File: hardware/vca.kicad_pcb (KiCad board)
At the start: 2 copper layers, 76.2 x 109.2 mm, 93 parts, among them P1 VCA_CMD_PWR, P10 CARD_2, P11 OUT_MAIN, P12 OUT_GND, P2 CARD_0, P3 CARD_1, P4 OUT_0, P5 OUT_1, P6 OUT_2, P7 OUT_3, P8 OUT_4, P9 OUT_5, U1 TL074, U10 TL082, U2 TL082, U3 4051, U4 SSM2164, U5 TL082, U6 TL082, U7 TL074, U8 SSM2164, U9 TL082

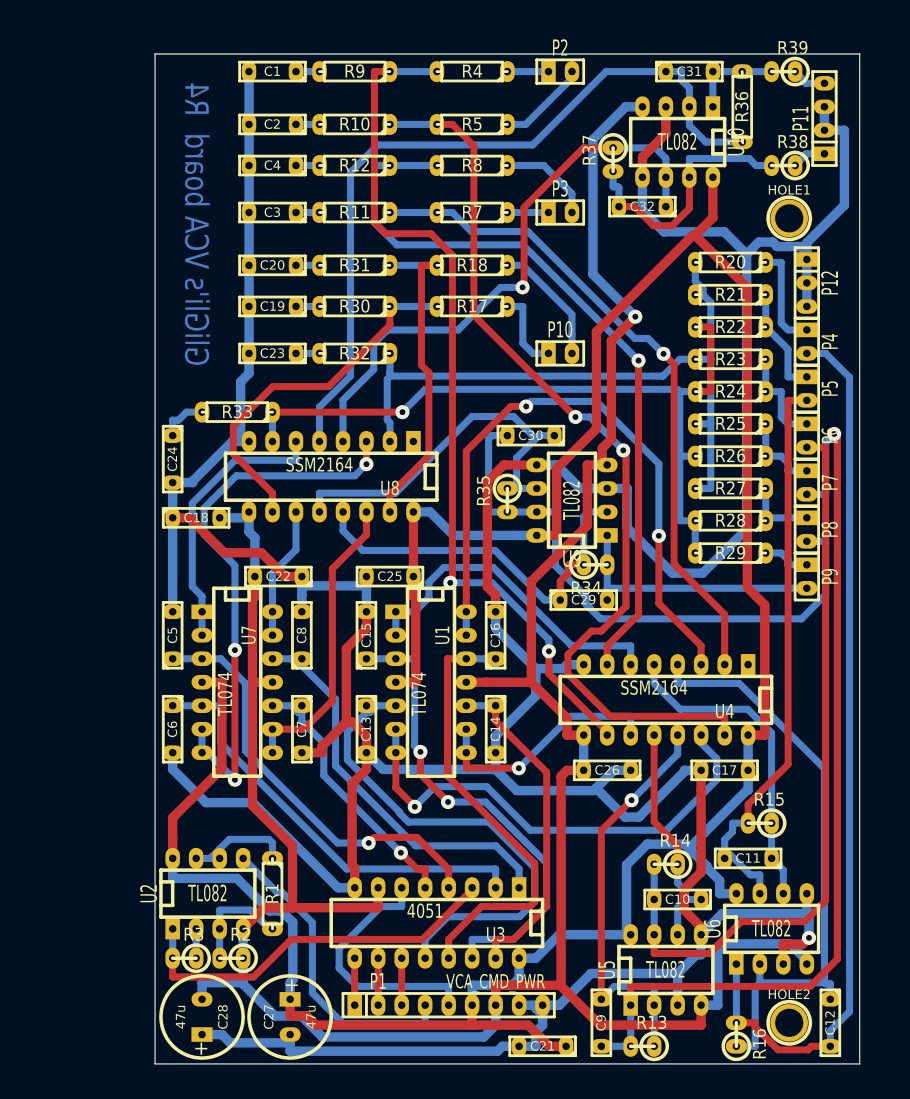
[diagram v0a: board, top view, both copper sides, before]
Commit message: hw: LM13700 vca board wip
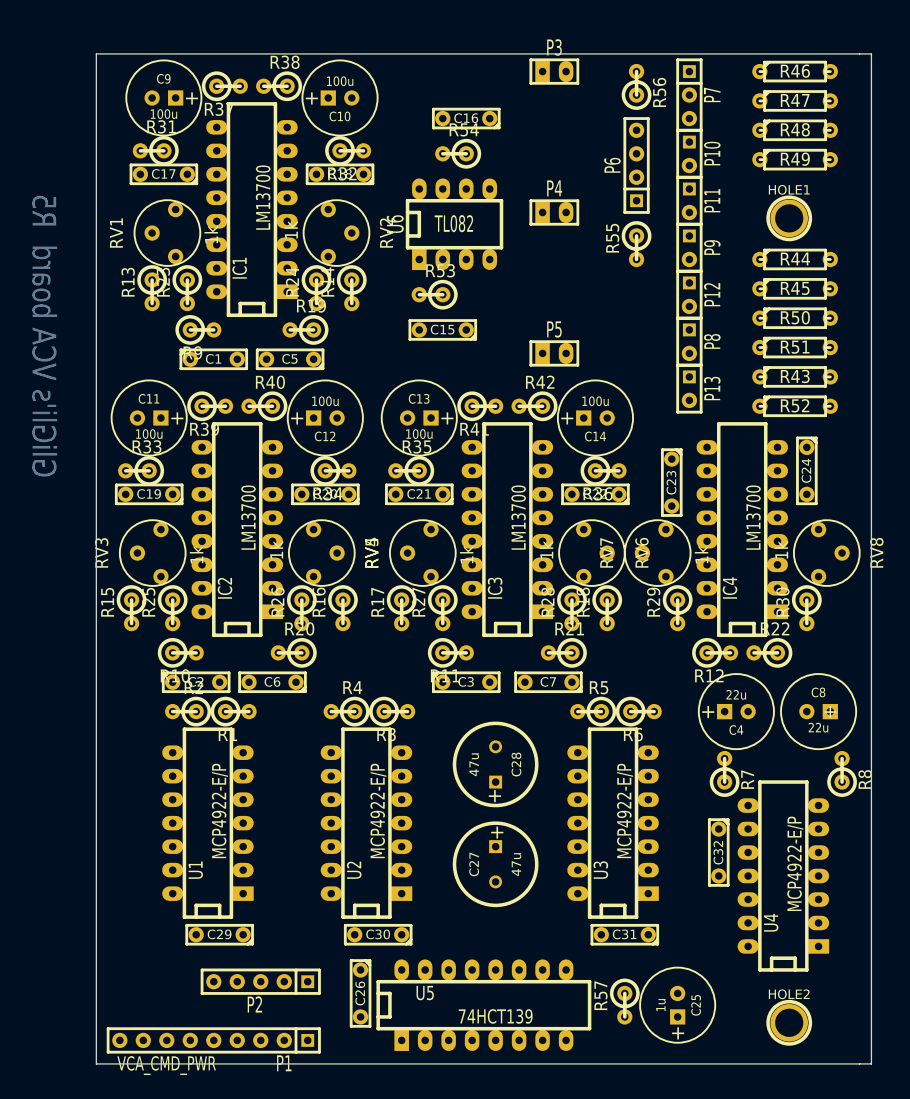
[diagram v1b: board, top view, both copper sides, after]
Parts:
- removed U10, U9: TL082, DIP-8__300_ELL
- removed U7: TL074, DIP-14__300_ELL
- removed U8: SSM2164, DIP-16__300_ELL
- added IC1: LM13700, DIP-16__300_ELL, F.Cu at (89.2, 67.6)
- added IC2: LM13700, DIP-16__300_ELL, F.Cu at (87.6, 102.2)
- added IC3: LM13700, DIP-16__300_ELL, F.Cu at (116.8, 102.2)
- added IC4: LM13700, DIP-16__300_ELL, F.Cu at (142.2, 102.2)
- added P13: OUT_5, SIL-2, F.Cu at (136.5, 87.0)
- added R19: 1k, R1, F.Cu at (94.6, 80.6)
- added R40: 4k7, R1, F.Cu at (90.2, 88.9)
- added R41: 4k7, R1, F.Cu at (114.3, 88.9)
- added R42: 4k7, R1, F.Cu at (119.4, 88.9)
- added R43: 33k, R3-LARGE_PADS, F.Cu at (148.0, 85.7)
- added R44: 47k, R3-LARGE_PADS, F.Cu at (148.0, 73.0)
- added R45: 150k, R3-LARGE_PADS, F.Cu at (148.0, 76.2)
- added R46: 56k, R3-LARGE_PADS, F.Cu at (148.0, 52.7)
- added R47: 68k, R3-LARGE_PADS, F.Cu at (148.0, 55.9)
- added R48: 68k, R3-LARGE_PADS, F.Cu at (148.0, 59.1)
- added R49: 56k, R3-LARGE_PADS, F.Cu at (148.0, 62.2)
- added R50: 150k, R3-LARGE_PADS, F.Cu at (148.0, 79.4)
- added R51: 47k, R3-LARGE_PADS, F.Cu at (148.0, 82.5)
- added R52: 33k, R3-LARGE_PADS, F.Cu at (148.0, 88.9)
- added R53: 47k, R1, F.Cu at (108.6, 76.8)
- added R54: 47k, R1, F.Cu at (111.1, 61.6)
- added R55: 1k, R1, F.Cu at (130.8, 71.8)
- added R56: 1k, R1, F.Cu at (130.8, 54.0)
- added R57: 100k, R1, F.Cu at (129.5, 153.7)
- added R6: 4k7, R1, F.Cu at (131.4, 121.9)
- added RV1: 1k, RV2, F.Cu at (79.7, 70.2)
- added RV2: 1k, RV2, F.Cu at (98.7, 70.2)
- added RV3: 1k, RV2, F.Cu at (78.1, 104.8)
- added RV4: 1k, RV2, F.Cu at (97.2, 104.8)
- added RV5: 1k, RV2, F.Cu at (107.3, 104.8)
- added RV6: 1k, RV2, F.Cu at (126.4, 104.8)
- added RV7: 1k, RV2, F.Cu at (132.7, 104.8)
- added RV8: 1k, RV2, F.Cu at (151.8, 104.8)
- C1, C2, C3: value 470p -> 470n
- C10, C11, C12, C9: value 100p -> 100u; footprint C2 -> C1V8
- C13, C14: value 47n -> 100u; footprint C2 -> C1V8
- C15, C16: value 47n -> 100p
- C19, C20, C23, C24: value 470p -> 100n
- C25: value 100n -> 1u; footprint C2 -> C1V8
- C29, C30, C31, C32: value 100p -> 100n
- C4: value 470p -> 22u; footprint C2 -> C1V8
- C5, C6, C7: value 47n -> 470n
- C8: value 47n -> 22u; footprint C2 -> C1V8
- P10: value CARD_2 -> OUT_0
- P11: value OUT_MAIN -> OUT_1; footprint SIL-4 -> SIL-2
- P12: value OUT_GND -> OUT_3; footprint SIL-3 -> SIL-2
- P2: value CARD_0 -> VCA_SPI; footprint SIL-2 -> SIL-5
- P3: value CARD_1 -> CARD_01
- P4: value OUT_0 -> CARD_23
- P5: value OUT_1 -> CARD_45
- P6: value OUT_2 -> OUT_MAIN; footprint SIL-2 -> SIL-4
- P7: value OUT_3 -> OUT_GND; footprint SIL-2 -> SIL-3
- P9: value OUT_5 -> OUT_2
- R1: value 10k -> 4k7; footprint R3-LARGE_PADS -> R1
- R10, R11, R12, R9: value 470 -> 1k; footprint R3-LARGE_PADS -> R1
- R17, R18: value 33k -> 10k; footprint R3-LARGE_PADS -> R1
- R2: value 82k -> 4k7
- R20: value 33k -> 1k; footprint R3-LARGE_PADS -> R1
- R21: value 47k -> 1k; footprint R3-LARGE_PADS -> R1
- R22: value 150k -> 1k; footprint R3-LARGE_PADS -> R1
- R23, R26: value 56k -> 6k8; footprint R3-LARGE_PADS -> R1
- R24, R25: value 68k -> 6k8; footprint R3-LARGE_PADS -> R1
- R27: value 150k -> 6k8; footprint R3-LARGE_PADS -> R1
- R28: value 47k -> 6k8; footprint R3-LARGE_PADS -> R1
- R29: value 33k -> 6k8; footprint R3-LARGE_PADS -> R1
- R3, R37: value 10k -> 4k7
- R30: value 470 -> 6k8; footprint R3-LARGE_PADS -> R1
- R31, R32, R33: value 470 -> 33k; footprint R3-LARGE_PADS -> R1
- R34, R35: value 10k -> 33k
- R36: value 10k -> 33k; footprint R3-LARGE_PADS -> R1
- R38, R39: value 1k -> 4k7
- R4, R5, R7, R8: value 33k -> 4k7; footprint R3-LARGE_PADS -> R1
- U1: value TL074 -> MCP4922-E/P
- U2: value TL082 -> MCP4922-E/P; footprint DIP-8__300_ELL -> DIP-14__300_ELL
- U3: value 4051 -> MCP4922-E/P; footprint DIP-16__300_ELL -> DIP-14__300_ELL
- U4: value SSM2164 -> MCP4922-E/P; footprint DIP-16__300_ELL -> DIP-14__300_ELL
- U5: value TL082 -> 74HCT139; footprint DIP-8__300_ELL -> DIP-16__300_ELL
- moved C9 110.6 mm to (79.7, 55.6), turned to 180 degrees
- moved P2 104.0 mm to (88.9, 151.1), turned to 180 degrees
- moved R13 97.3 mm to (78.4, 76.5), turned to 270 degrees
- moved C10 94.1 mm to (98.7, 55.6), turned to 0 degrees
- moved C31 93.6 mm to (129.5, 146.1), turned to 180 degrees
- moved C17 88.5 mm to (79.7, 63.8)
- moved C12 85.2 mm to (97.2, 90.2), turned to 0 degrees
- moved U6 83.6 mm to (111.1, 69.2)
- moved C11 80.4 mm to (78.1, 90.2)
- moved C4 77.5 mm to (141.6, 121.9), turned to 0 degrees
- moved R8 76.7 mm to (153.0, 128.3), turned to 90 degrees
- moved R15 71.7 mm to (76.2, 111.1), turned to 270 degrees
- moved R39 71.4 mm to (85.1, 88.9), turned to 0 degrees
- moved R14 70.6 mm to (100.0, 76.5), turned to 270 degrees
- moved R4 70.6 mm to (99.1, 121.9)
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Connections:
- C1 pad 1: N-0000059 -> N-0000098
- C1 pad 2: GND -> -5V
- C10 pad 1: N-0000055 -> N-0000096
- C10 pad 2: N-0000074 -> N-0000045
- C11 pad 1: N-0000051 -> N-0000021
- C11 pad 2: N-0000072 -> N-0000044
- C12 pad 1: N-0000056 -> N-0000027
- C12 pad 2: N-0000057 -> N-0000043
- C13 pad 1: N-0000020 -> N-0000016
- C13 pad 2: GND -> N-0000049
- C14 pad 1: N-0000011 -> N-0000015
- C14 pad 2: GND -> N-0000048
- C15 pad 1: N-000009 -> N-0000041
- C15 pad 2: GND -> N-0000065
- C16 pad 1: N-0000046 -> N-0000040
- C16 pad 2: GND -> N-0000067
- C19 pad 1: N-0000036 -> +5V
- C2 pad 1: N-0000058 -> N-0000020
- C2 pad 2: GND -> -5V
- C20 pad 1: N-0000035 -> GND
- C20 pad 2: GND -> -5V
- C23 pad 1: N-0000070 -> +5V
- C24 pad 1: N-0000068 -> GND
- C24 pad 2: GND -> -5V
- C25 pad 1: +5V -> VAA
- C26 pad 1: GND -> +5V
- C26 pad 2: -5V -> GND
- C29 pad 1: N-0000043 -> +5V
- C29 pad 2: N-0000021 -> GND
- C3 pad 1: N-0000013 -> N-0000019
- C3 pad 2: GND -> -5V
- C30 pad 1: N-0000045 -> +5V
- C30 pad 2: N-0000022 -> GND
- C31 pad 1: N-0000023 -> +5V
- C31 pad 2: N-0000032 -> GND
- C32 pad 1: N-0000033 -> +5V
- C32 pad 2: N-0000034 -> GND
- C4 pad 1: N-0000012 -> N-0000058
- C4 pad 2: GND -> -5V
- C5 pad 1: N-0000016 -> N-0000072
- C5 pad 2: GND -> -5V
- C6 pad 1: N-0000017 -> N-0000023
- C6 pad 2: GND -> -5V
- C7 pad 1: N-0000018 -> N-0000012
- C7 pad 2: GND -> -5V
- C8 pad 1: N-0000019 -> N-0000064
- C8 pad 2: GND -> -5V
- C9 pad 1: N-0000047 -> N-0000097
- C9 pad 2: N-0000048 -> N-0000042
- P1 pad 1: N-000002 -> (no net)
- P1 pad 2: N-000001 -> N-0000056
- P1 pad 3: N-000003 -> N-0000050
- P1 pad 4: N-0000031 -> (no net)
- P1 pad 5: N-000004 -> N-0000055
- P10 pad 1: N-0000037 -> N-0000075
- P10 pad 2: N-0000038 -> N-0000042
- P11 pad 1: N-0000041 -> N-0000073
- P11 pad 2: GND -> N-0000045
- P12 pad 1: GND -> N-0000076
- P12 pad 2: GND -> N-0000043
- P2 pad 1: N-0000060 -> N-0000087
- P2 pad 2: N-0000061 -> N-0000086
- P3 pad 1: N-0000014 -> N-0000092
- P3 pad 2: N-0000015 -> N-0000091
- P4 pad 1: N-0000064 -> N-0000031
- P4 pad 2: N-0000057 -> N-0000030
- P5 pad 1: N-0000071 -> N-000004
- P5 pad 2: N-0000072 -> N-000003
- P6 pad 1: N-0000073 -> N-0000077
- P6 pad 2: N-0000074 -> GND
- P7 pad 1: N-0000075 -> GND
- P7 pad 2: N-0000048 -> GND
- P8 pad 1: N-0000063 -> N-0000068
- P8 pad 2: N-0000022 -> N-0000049
- P9 pad 1: N-0000066 -> N-0000074
- P9 pad 2: N-0000021 -> N-0000044
- R1 pad 1: N-0000029 -> N-0000082
- R1 pad 2: N-0000044 -> N-0000098
- R10 pad 1: N-000006 -> N-0000020
- R10 pad 2: N-0000058 -> -5V
- R11 pad 1: N-000008 -> N-0000019
- R11 pad 2: N-0000013 -> -5V
- R12 pad 1: N-000007 -> N-0000058
- R12 pad 2: N-0000012 -> -5V
- R13 pad 1: N-0000047 -> N-0000088
- R13 pad 2: N-0000048 -> N-0000092
- R14 pad 1: N-0000055 -> N-00000100
- R14 pad 2: N-0000074 -> N-0000091
- R15 pad 1: N-0000051 -> N-0000094
- R15 pad 2: N-0000072 -> N-0000031
- R16 pad 1: N-0000056 -> N-0000093
- R16 pad 2: N-0000057 -> N-0000030
- R17 pad 1: N-0000037 -> N-000008
- R17 pad 2: N-0000027 -> N-000004
- R18 pad 1: N-0000038 -> N-000005
- R18 pad 2: N-0000026 -> N-000003
- R2 pad 1: -5V -> N-0000081
- R2 pad 2: N-0000044 -> N-0000072
- R20 pad 1: N-0000064 -> N-0000023
- R20 pad 2: N-0000069 -> -5V
- R21 pad 1: N-0000071 -> N-0000012
- R21 pad 2: N-0000069 -> -5V
- R22 pad 1: N-0000071 -> N-0000064
- R22 pad 2: N-0000076 -> -5V
- R23 pad 1: N-0000073 -> N-0000095
- R23 pad 2: N-0000069 -> +5V
- R24 pad 1: N-0000073 -> N-0000071
- R24 pad 2: N-0000076 -> +5V
- R25 pad 1: N-0000075 -> N-0000090
- R25 pad 2: N-0000069 -> +5V
- R26 pad 1: N-0000075 -> N-0000025
- R26 pad 2: N-0000076 -> +5V
- R27 pad 1: N-0000063 -> N-000002
- R27 pad 2: N-0000069 -> +5V
- R28 pad 1: N-0000063 -> N-000009
- R28 pad 2: N-0000076 -> +5V
- R29 pad 1: N-0000066 -> N-0000059
- R29 pad 2: N-0000076 -> +5V
- R3 pad 1: N-0000039 -> N-0000032
- R3 pad 2: N-0000030 -> N-0000020
- R30 pad 1: N-0000027 -> N-0000038
- R30 pad 2: N-0000036 -> +5V
- R31 pad 1: N-0000026 -> N-0000099
- R31 pad 2: N-0000035 -> GND
- R32 pad 1: N-0000069 -> N-00000101
- R32 pad 2: N-0000070 -> GND
- R33 pad 1: N-0000076 -> N-0000022
- R33 pad 2: N-0000068 -> GND
- R34 pad 1: N-0000043 -> N-0000028
- R34 pad 2: N-0000021 -> GND
- R35 pad 1: N-0000045 -> N-0000017
- R35 pad 2: N-0000022 -> GND
- R36 pad 1: N-0000023 -> N-0000018
- R36 pad 2: N-0000032 -> GND
- R37 pad 1: N-0000033 -> N-0000097
- R37 pad 2: N-0000034 -> -5V
- R38 pad 1: N-0000041 -> N-0000096
- R38 pad 2: N-0000034 -> -5V
- R39 pad 1: N-0000042 -> N-0000021
- R39 pad 2: N-0000032 -> -5V
- R4 pad 1: N-0000060 -> N-0000033
- R4 pad 2: N-000005 -> N-0000023
- R5 pad 1: N-0000061 -> N-0000014
- R5 pad 2: N-000006 -> N-0000019
- R7 pad 1: N-0000014 -> N-0000062
- R7 pad 2: N-000008 -> N-0000058
- R8 pad 1: N-0000015 -> N-0000063
- R8 pad 2: N-000007 -> N-0000064
- R9 pad 1: N-000005 -> N-0000098
- R9 pad 2: N-0000059 -> -5V
- U1 pad 1: N-0000053 -> +5V
- U1 pad 10: N-0000011 -> N-0000081
- U1 pad 11: -5V -> VAA
- U1 pad 12: N-0000046 -> GND
- U1 pad 13: N-0000054 -> VAA
- U1 pad 14: N-0000054 -> N-0000082
- U1 pad 2: N-0000053 -> (no net)
- U1 pad 3: N-000009 -> N-0000085
- U1 pad 4: +5V -> N-0000086
- U1 pad 5: N-0000020 -> N-0000087
- U1 pad 6: N-0000010 -> (no net)
- U1 pad 7: N-0000010 -> (no net)
- U1 pad 8: N-0000052 -> N-0000047
- U1 pad 9: N-0000052 -> +5V
- U2 pad 1: N-0000030 -> +5V
- U2 pad 2: N-0000039 -> (no net)
- U2 pad 3: N-0000044 -> N-0000085
- U2 pad 4: -5V -> N-0000086
- U2 pad 5: N-0000031 -> N-0000087
- U2 pad 6: N-0000029 -> (no net)
- U2 pad 7: N-0000029 -> (no net)
- U2 pad 8: +5V -> N-0000046
- U3 pad 1: N-0000019 -> +5V
- U3 pad 10: N-000001 -> N-0000013
- U3 pad 11: N-000003 -> VAA
- U3 pad 12: N-0000020 -> GND
- U3 pad 13: N-0000046 -> VAA
- U3 pad 14: N-000009 -> N-0000014
- U3 pad 2: N-0000017 -> (no net)
- U3 pad 3: N-0000030 -> N-0000085
- U3 pad 4: N-0000016 -> N-0000086
- U3 pad 5: N-0000018 -> N-0000087
- U3 pad 6: N-000004 -> (no net)
- U3 pad 7: -5V -> (no net)
- U3 pad 8: GND -> N-0000034
- U3 pad 9: N-000002 -> +5V
- U4 pad 1: (no net) -> +5V
- U4 pad 10: N-000005 -> N-0000063
- U4 pad 11: N-0000052 -> VAA
- U4 pad 12: N-0000055 -> GND
- U4 pad 13: N-0000047 -> VAA
- U4 pad 14: N-0000010 -> N-0000062
- U4 pad 2: N-000008 -> (no net)
- U4 pad 3: N-0000054 -> N-0000085
- U4 pad 4: N-0000056 -> N-0000086
- U4 pad 5: N-0000051 -> N-0000087
- U4 pad 6: N-0000053 -> (no net)
- U4 pad 7: N-000007 -> (no net)
- U4 pad 8: GND -> N-0000039
- U4 pad 9: -5V -> +5V
- U5 pad 1: N-0000048 -> N-0000055
- U5 pad 2: N-0000047 -> N-0000050
- U5 pad 3: GND -> N-0000056
- U5 pad 4: -5V -> N-0000047
- U5 pad 5: GND -> N-0000046
- U5 pad 6: N-0000055 -> N-0000034
- U5 pad 7: N-0000074 -> N-0000039
- U5 pad 8: +5V -> GND
- U6 pad 1: N-0000057 -> N-0000065
- U6 pad 2: N-0000056 -> N-0000041
- U6 pad 6: N-0000051 -> N-0000040
- U6 pad 7: N-0000072 -> N-0000067
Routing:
- net GND: track 487.8 -> 0.00 mm, vias 1 -> 0
- net +5V: track 287.5 -> 0.00 mm
- net -5V: track 278.6 -> 0.00 mm, vias 1 -> 0
- net N-0000048: track 99.1 -> 0.00 mm, vias 1 -> 0
- net N-000006: track 99.0 -> 0.00 mm, vias 2 -> 0
- net N-0000057: track 97.1 -> 0.00 mm
- net N-000005: track 94.6 -> 0.00 mm, vias 2 -> 0
- net N-0000023: track 83.5 -> 0.00 mm
- net N-000007: track 82.0 -> 0.00 mm, vias 1 -> 0
- net N-0000074: track 81.6 -> 0.00 mm
- net N-0000076: track 81.2 -> 0.00 mm, vias 1 -> 0
- net N-0000069: track 74.5 -> 0.00 mm
- net N-000008: track 72.3 -> 0.00 mm, vias 1 -> 0
- net N-0000054: track 69.4 -> 0.00 mm, vias 2 -> 0
- net N-0000056: track 65.4 -> 0.00 mm
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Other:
- board size 76.2 x 109.2 mm -> 83.8 x 109.2 mm
- board text added: "GliGli's VCA board R5"
- board text removed: "GliGli's VCA board R4"
